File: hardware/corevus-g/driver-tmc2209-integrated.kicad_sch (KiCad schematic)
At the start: 12 parts, among them M1 JST XH, U6 TMC2209-LA

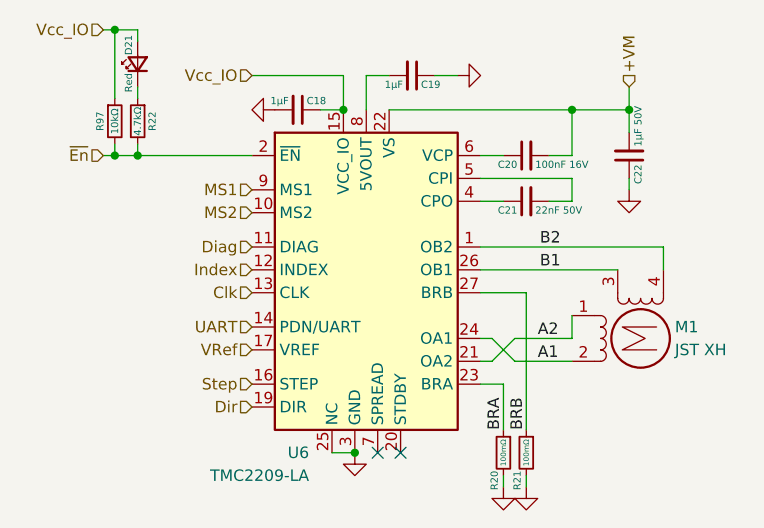
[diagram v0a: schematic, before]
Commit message: why not
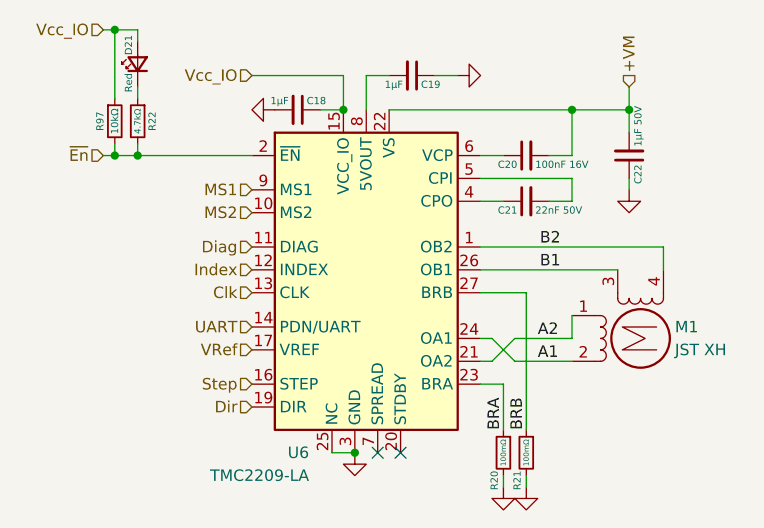
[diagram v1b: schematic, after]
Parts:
- C20: LCSC C1525 -> (none)
- C21: LCSC C1532 -> (none)
- C22: LCSC C15849 -> (none)
- R20, R21: LCSC C382279 -> (none)
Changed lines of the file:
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@@
-			)
-		)
-		(property "LCSC" "C1532"
-			(at 82.55 58.42 90)
-			(effects
-				(font
-					(size 1.27 1.27)
-				)
-				(hide yes)
 			)
 		)
@@
 			(effects
 				(font
-					(size 0.8 0.8)
+					(size 0.7 0.7)
 				)
 			)
@@
 			)
 		)
-		(property "LCSC" "C382279"
-			(at 80.01 86.36 90)
-			(effects
-				(font
-					(size 1.27 1.27)
-				)
-				(hide yes)
-			)
-		)
 		(pin "1"
 		)
@@
 			)
 		)
-		(property "LCSC" "C1525"
-			(at 82.55 53.34 90)
-			(effects
-				(font
-					(size 1.27 1.27)
-				)
-				(hide yes)
-			)
-		)
 		(pin "1"
 		)
@@
 		(property "Description" ""
 			(at 93.98 53.34 0)
-			(effects
-				(font
-					(size 1.27 1.27)
-				)
-				(hide yes)
-			)
-		)
-		(property "LCSC" "C15849"
-			(at 93.98 53.34 90)
 			(effects
 				(font
@@
 			(effects
 				(font
-					(size 1.27 1.27)
-				)
-				(hide yes)
-			)
-		)
-		(property "LCSC" "C382279"
-			(at 82.55 86.36 90)
-			(effects
-				(font
